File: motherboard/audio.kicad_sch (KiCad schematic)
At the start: 1 part, among them U23 TPA2028D1YZFT

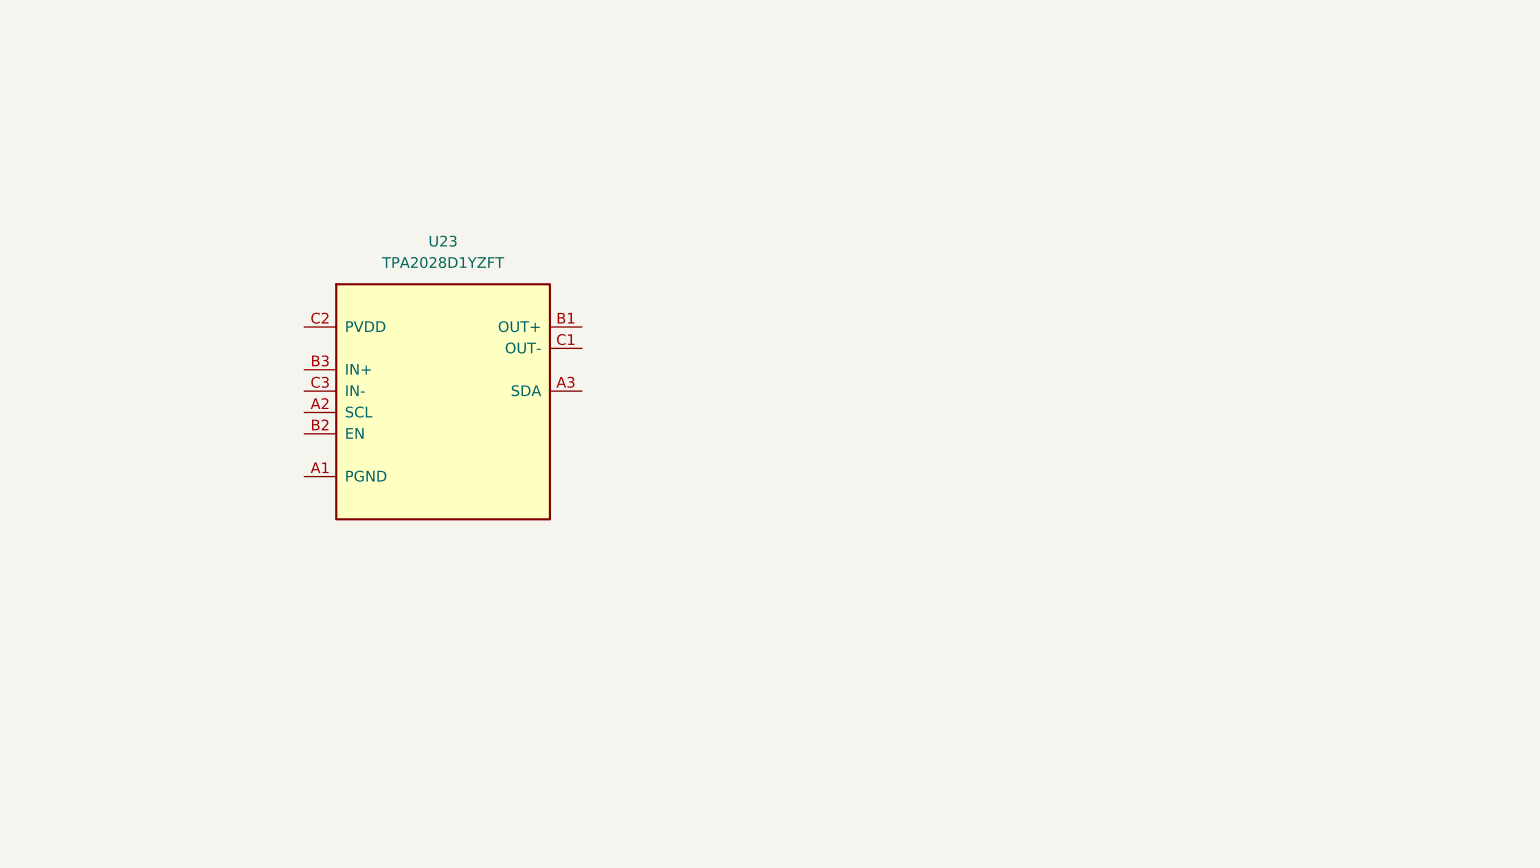
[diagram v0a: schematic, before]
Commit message: audio done
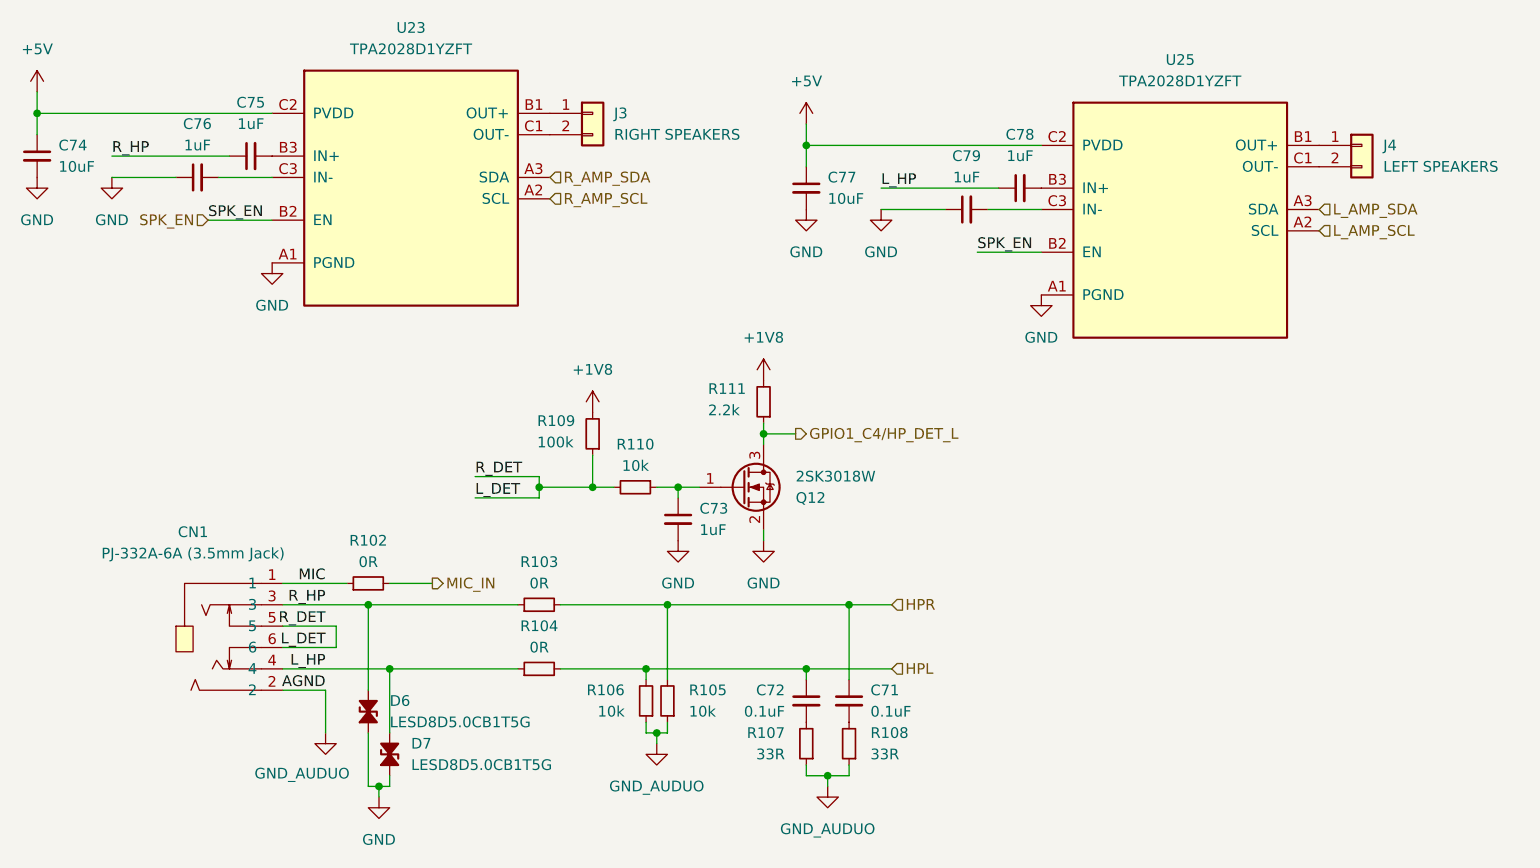
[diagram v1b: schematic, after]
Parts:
- added C71, C72: 0.1uF, Capacitor_SMD:C_0402_1005Metric, symbol Device:C_Small
- added C73, C75, C76, C78, C79: 1uF, Capacitor_SMD:C_0402_1005Metric, symbol Device:C_Small
- added C74, C77: 10uF, Capacitor_SMD:C_0402_1005Metric, symbol Device:C_Small
- added CN1: PJ-332A-6A (3.5mm Jack), Headphone_Jack:AUDIO-SMD_PJ-332A-6A, symbol Headphone_Jack:PJ-332A-6A
- added D6, D7: LESD8D5.0CB1T5G, Diode_SMD:D_SOD-882, symbol Device:D_TVS_Small_Filled
- added J3: RIGHT SPEAKERS, symbol Connector_Generic:Conn_01x02
- added J4: LEFT SPEAKERS, symbol Connector_Generic:Conn_01x02
- added Q12: 2SK3018W, Package_TO_SOT_SMD:SOT-323_SC-70, symbol Transistor_FET:BSS214NW
- added R102, R103, R104: 0R, Resistor_SMD:R_0402_1005Metric, symbol Device:R_Small
- added R105, R106, R110: 10k, Resistor_SMD:R_0402_1005Metric, symbol Device:R_Small
- added R107, R108: 33R, Resistor_SMD:R_0402_1005Metric, symbol Device:R_Small
- added R109: 100k, Resistor_SMD:R_0402_1005Metric, symbol Device:R_Small
- added R111: 2.2k, Resistor_SMD:R_0402_1005Metric, symbol Device:R_Small
- added U25: TPA2028D1YZFT, TPA2028D1YZFT:BGA9C50P3X3_162X162X63, symbol Audio_Amp:TPA2028D1YZFT
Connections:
- net GND: now reaches U23.A1 (PGND)
- net GND: now also C73.2, C74.2, C76.1, C77.2, C79.1, D6.1 (A1), D7.1 (A1), Q12.2 (S), U25.A1 (PGND)
- net R_AMP_SCL: now reaches U23.A2 (SCL)
- net R_AMP_SDA: now reaches U23.A3 (SDA)
- net at U23.B1 (OUT+): now also J3.1 (Pin_1)
- net SPK_EN: now reaches U23.B2 (EN)
- net SPK_EN: now also U25.B2 (EN)
- net at U23.B3 (IN+): now also C75.2
- net at U23.C1 (OUT-): now also J3.2 (Pin_2)
- net +5V: now reaches U23.C2 (PVDD)
- net +5V: now also C74.1, C77.1, U25.C2 (PVDD)
- net at U23.C3 (IN-): now also C76.2
- new net: C72.2, R107.2
- new net: C73.1, Q12.1 (G), R110.1
- new net: J4.1 (Pin_1), U25.B1 (OUT+)
- new net: C78.2, U25.B3 (IN+)
- new net: J4.2 (Pin_2), U25.C1 (OUT-)
- new net: C79.2, U25.C3 (IN-)
- new net: C71.2, R108.2
- new net +1V8: R109.2, R111.2
- new net GND_AUDUO: CN1.2, R105.1, R106.1, R107.1, R108.1
- new net GPIO1_C4/HP_DET_L: Q12.3 (D), R111.1
- new net HPL: C72.1, R104.2, R106.2
- new net HPR: C71.1, R103.2, R105.2
- new net L_AMP_SCL: U25.A2 (SCL)
- new net L_AMP_SDA: U25.A3 (SDA)
- new net L_DET: CN1.5, CN1.6, R109.1, R110.2
- new net L_HP: C78.1, CN1.4, D7.2 (A2), R104.1
- new net MIC: CN1.1, R102.1
- new net MIC_IN: R102.2
- new net R_HP: C75.1, CN1.3, D6.2 (A2), R103.1
